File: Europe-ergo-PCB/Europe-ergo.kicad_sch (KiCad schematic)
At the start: 230 parts, among them J1 Conn_01x04_Male/I2C, J2 Conn_01x04_Male, SW1 MX-NO-LED, SW10 MX-NO-LED, SW11 MX-NO-LED, SW12 MX-NO-LED, SW13 MX-NO-LED, SW14 MX-NO-LED, SW15 MX-NO-LED, SW16 MX-NO-LED, SW17 MX-NO-LED, SW18 MX-NO-LED, SW19 MX-NO-LED, SW2 MX-NO-LED, SW20 MX-NO-LED, SW21 MX-NO-LED, SW22 MX-NO-LED, SW23 MX-NO-LED, SW24 MX-NO-LED, SW25 MX-NO-LED, SW26 MX-NO-LED, SW27 MX-NO-LED, SW28 MX-NO-LED, SW29 MX-NO-LED, SW3 MX-NO-LED, SW30 MX-NO-LED, SW31 MX-NO-LED, SW32 MX-NO-LED, SW33 MX-NO-LED, SW34 MX-NO-LED, SW35 MX-NO-LED, SW36 MX-NO-LED, SW37 MX-NO-LED, SW38 MX-NO-LED, SW39 MX-NO-LED, SW4 MX-NO-LED, SW40 MX-NO-LED, SW41 MX-NO-LED, SW42 MX-NO-LED, SW43 MX-NO-LED, SW44 MX-NO-LED, SW45 MX-NO-LED, SW46 MX-NO-LED, SW47 MX-NO-LED, SW48 SW_Push, SW49 SW_Push, SW5 MX-NO-LED, SW50 MX-NO-LED, SW51 MX-NO-LED, SW52 MX-NO-LED, SW53 MX-NO-LED, SW54 MX-NO-LED, SW55 MX-NO-LED, SW56 MX-NO-LED, SW57 MX-NO-LED, SW58 MX-NO-LED, SW59 MX-NO-LED, SW6 MX-NO-LED, SW60 MX-NO-LED, SW61 MX-NO-LED, SW62 MX-NO-LED, SW63 MX-NO-LED, SW64 MX-NO-LED, SW65 MX-NO-LED, SW66 MX-NO-LED, SW67 MX-NO-LED, SW68 MX-NO-LED, SW69 MX-NO-LED, SW7 MX-NO-LED, SW70 MX-NO-LED, SW71 MX-NO-LED, SW72 MX-NO-LED, SW73 MX-NO-LED, SW74 MX-NO-LED, SW75 MX-NO-LED, SW76 MX-NO-LED, SW77 MX-NO-LED, SW78 MX-NO-LED, SW79 MX-NO-LED, SW8 MX-NO-LED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

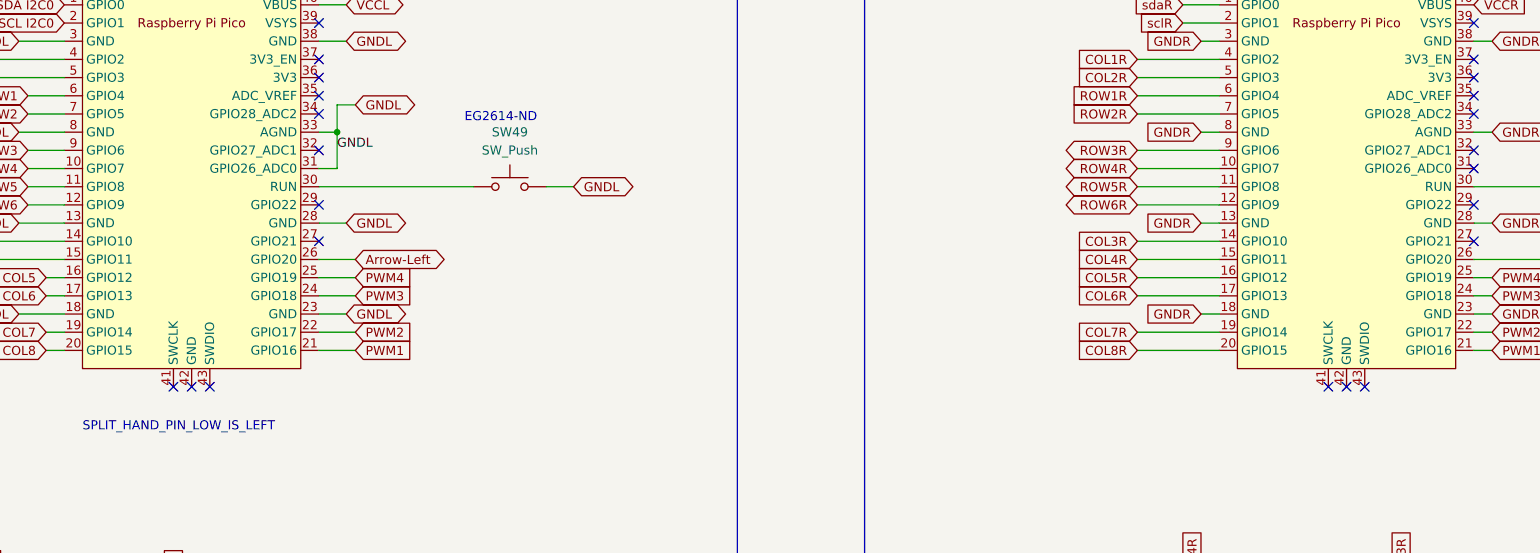
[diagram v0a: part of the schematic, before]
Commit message: Add files via upload
small fix
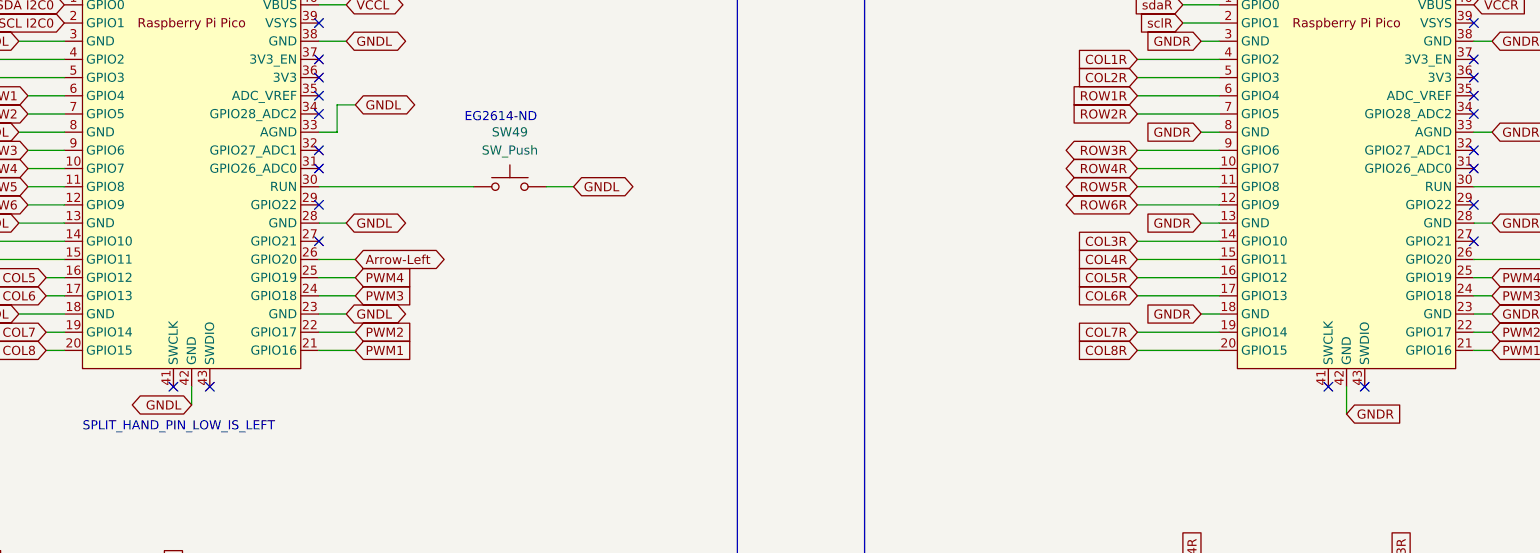
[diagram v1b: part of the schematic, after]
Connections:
- net GNDL: now also U2.42 (GND); no longer U2.31 (GPIO26_ADC0)
- net GNDR: now also U1.42 (GND)
- no-connect marks 23 -> 22
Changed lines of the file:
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@@
   (junction (at 722.63 241.3) (diameter 0) (color 0 0 0 0)
-  )
-  (junction (at 344.17 58.42) (diameter 0) (color 0 0 0 0)
   )
   (junction (at 759.46 223.52) (diameter 0) (color 0 0 0 0)
@@
   (no_connect (at 341.63 48.26))
   (no_connect (at 321.31 93.98))
-  (no_connect (at 323.85 93.98))
   (no_connect (at 502.92 48.26))
   (no_connect (at 502.92 53.34))
@@
   (no_connect (at 341.63 50.8))
   (no_connect (at 482.6 93.98))
-  (no_connect (at 485.14 93.98))
+  (no_connect (at 341.63 63.5))
   (no_connect (at 502.92 73.66))
   (no_connect (at 341.63 53.34))
@@
     (stroke (width 0) (type default) (color 0 0 0 0))
   )
-  (wire (pts (xy 341.63 63.5) (xy 344.17 63.5))
-    (stroke (width 0) (type default) (color 0 0 0 0))
-  )
   (wire (pts (xy 502.92 78.74) (xy 505.46 78.74))
     (stroke (width 0) (type default) (color 0 0 0 0))
@@
     (stroke (width 0) (type default) (color 0 0 0 0))
   )
-  (wire (pts (xy 344.17 58.42) (xy 344.17 63.5))
-    (stroke (width 0) (type default) (color 0 0 0 0))
-  )
   (wire (pts (xy 100.33 134.62) (xy 100.33 138.43))
     (stroke (width 0) (type default) (color 0 0 0 0))
@@
     (stroke (width 0) (type default) (color 0 0 0 0))
   )
+  (wire (pts (xy 485.14 93.98) (xy 485.14 97.79))
+    (stroke (width 0) (type default) (color 0 0 0 0))
+  )
   (wire (pts (xy 687.07 120.65) (xy 661.67 120.65))
     (stroke (width 0) (type default) (color 0 0 0 0))
@@
   )
   (wire (pts (xy 676.91 210.82) (xy 674.37 210.82))
+    (stroke (width 0) (type default) (color 0 0 0 0))
+  )
+  (wire (pts (xy 323.85 93.98) (xy 323.85 96.52))
     (stroke (width 0) (type default) (color 0 0 0 0))
   )
@@
     (effects (font (size 1.27 1.27)) (justify left bottom))
   )
-  (label "GNDL" (at 344.17 60.96 0)
-    (effects (font (size 1.27 1.27)) (justify left bottom))
-  )
   (label "RUN" (at 515.62 66.04 0)
     (effects (font (size 1.27 1.27)) (justify left bottom))
@@
     )
   )
+  (global_label "GNDR" (shape input) (at 485.14 97.79 0) (fields_autoplaced)
+    (effects (font (size 1.27 1.27)) (justify left))
+    (property "Intersheet References" "${INTERSHEET_REFS}" (id 0) (at 492.6047 97.7106 0)
+      (effects (font (size 1.27 1.27)) (justify left) hide)
+    )
+  )
   (global_label "VCCR" (shape input) (at 502.92 40.64 0) (fields_autoplaced)
     (effects (font (size 1.27 1.27)) (justify left))
@@
     )
   )
+  (global_label "GNDL" (shape bidirectional) (at 323.85 96.52 180) (fields_autoplaced)
+    (effects (font (size 1.27 1.27)) (justify right))
+    (property "Intersheet References" "${INTERSHEET_REFS}" (id 0) (at 316.5383 96.4406 0)
+      (effects (font (size 1.27 1.27)) (justify right) hide)
+    )
+  )

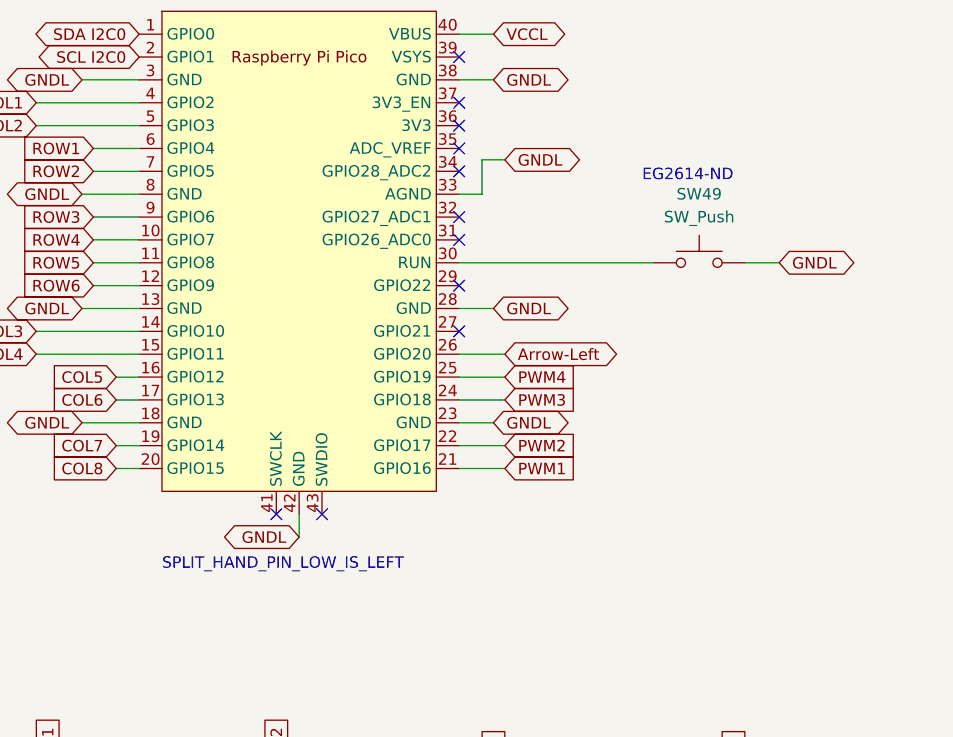
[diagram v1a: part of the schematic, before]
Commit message: Add files via upload
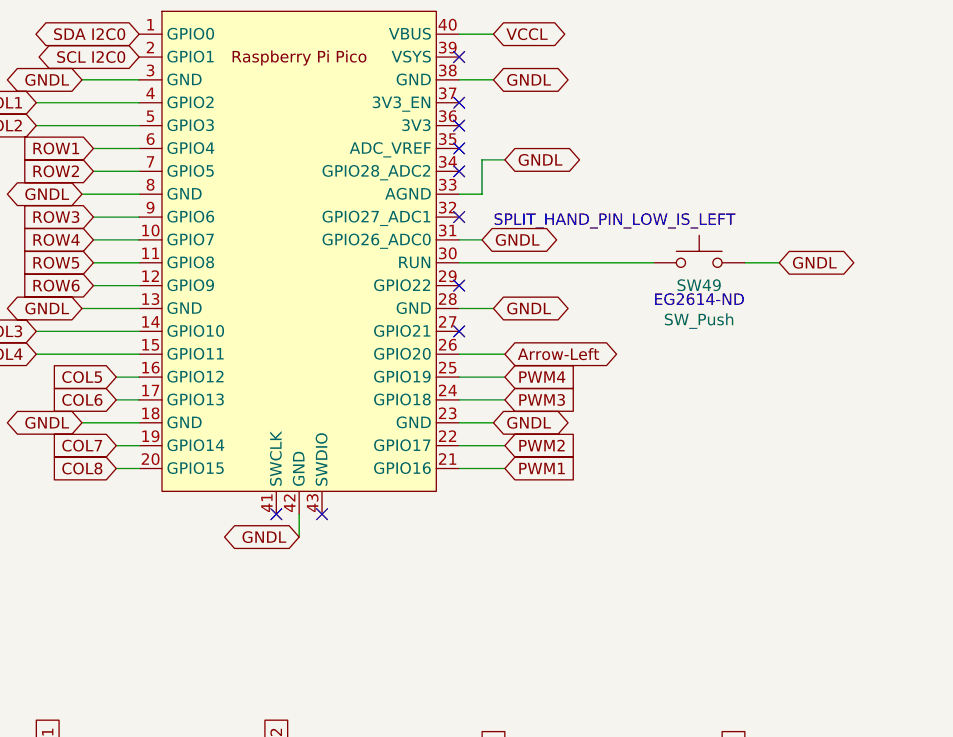
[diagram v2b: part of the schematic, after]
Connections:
- net GNDL: now also U2.31 (GPIO26_ADC0)
- no-connect marks 22 -> 21
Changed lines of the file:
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@@
   (no_connect (at 341.63 50.8))
   (no_connect (at 482.6 93.98))
-  (no_connect (at 341.63 63.5))
   (no_connect (at 502.92 73.66))
   (no_connect (at 341.63 53.34))
@@
     (stroke (width 0) (type default) (color 0 0 0 0))
   )
+  (wire (pts (xy 341.63 63.5) (xy 344.17 63.5))
+    (stroke (width 0) (type default) (color 0 0 0 0))
+  )
   (wire (pts (xy 651.51 100.33) (xy 651.51 138.43))
     (stroke (width 0) (type default) (color 0 0 0 0))
@@
     (stroke (width 0) (type default) (color 0 0 0 0))
   )
-  (text "EG2614-ND" (at 361.95 57.15 0)
+  (text "EG2614-ND" (at 363.22 71.12 0)
     (effects (font (size 1.27 1.27)) (justify left bottom))
   )
@@
     (effects (font (size 1.27 1.27)) (justify left bottom))
   )
-  (text "SPLIT_HAND_PIN_LOW_IS_LEFT" (at 308.61 100.33 0)
+  (text "SPLIT_HAND_PIN_LOW_IS_LEFT" (at 345.44 62.23 0)
     (effects (font (size 1.27 1.27)) (justify left bottom))
   )
@@
     )
   )
+  (global_label "GNDL" (shape bidirectional) (at 344.17 63.5 0) (fields_autoplaced)
+    (effects (font (size 1.27 1.27)) (justify left))
+    (property "Intersheet References" "${INTERSHEET_REFS}" (id 0) (at 351.4817 63.5794 0)
+      (effects (font (size 1.27 1.27)) (justify left) hide)
+    )
+  )
   (global_label "VCCR" (shape input) (at 513.08 196.85 0) (fields_autoplaced)
     (effects (font (size 1.27 1.27)) (justify left))
@@
   )
   (symbol (lib_id "Switch:SW_Push") (at 368.3 66.04 0) (unit 1)
-    (in_bom yes) (on_board yes) (fields_autoplaced)
-    (property "Reference" "SW49" (id 0) (at 368.3 58.42 0))
-    (property "Value" "SW_Push" (id 1) (at 368.3 60.96 0))
+    (in_bom yes) (on_board yes)
+    (property "Reference" "SW49" (id 0) (at 368.3 68.58 0))
+    (property "Value" "SW_Push" (id 1) (at 368.3 72.39 0))
     (property "Footprint" "switch:switch_P5.08mm" (id 2) (at 368.3 60.96 0)
       (effects (font (size 1.27 1.27)) hide)

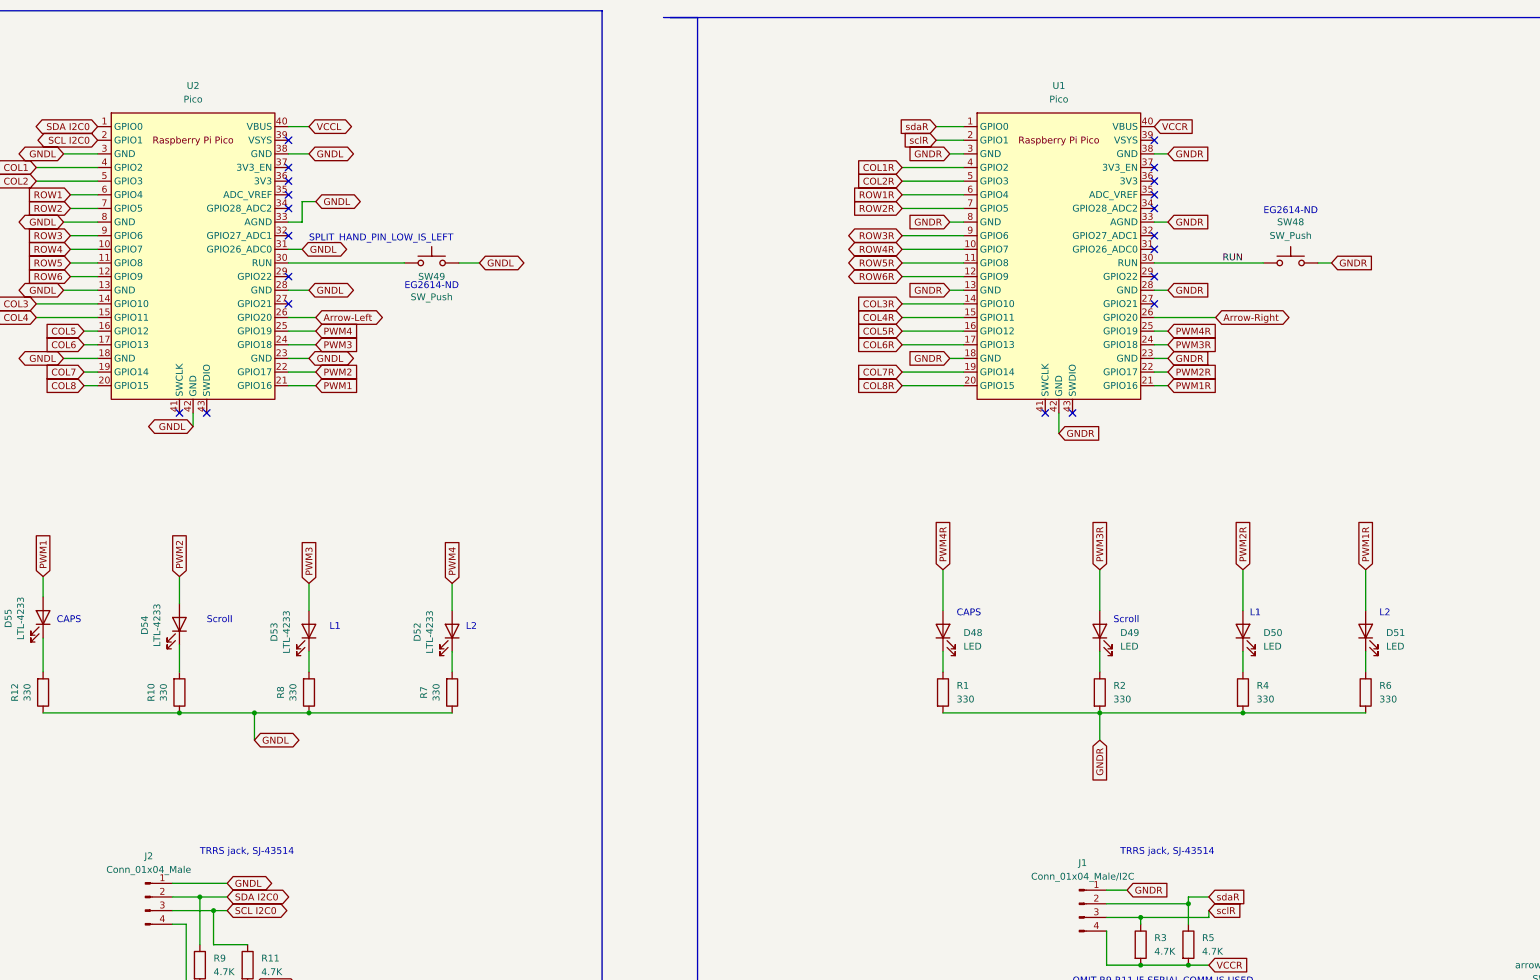
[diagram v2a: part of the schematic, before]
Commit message: Add files via upload
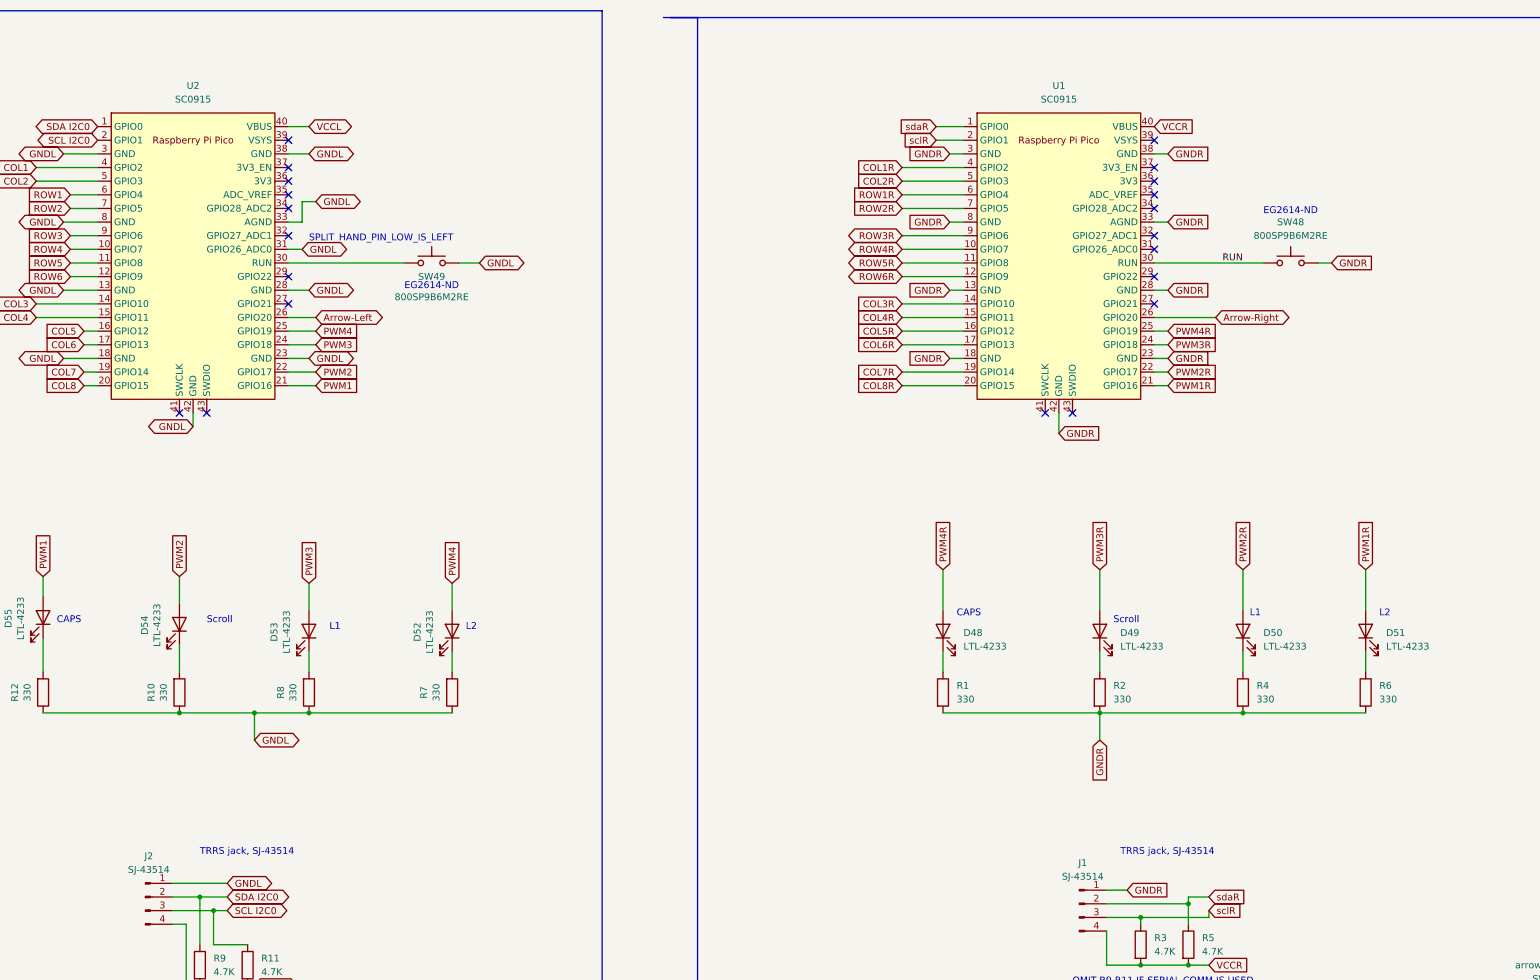
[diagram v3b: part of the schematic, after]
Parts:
- D48, D49, D50, D51: value LED -> LTL-4233
- J1: value Conn_01x04_Male/I2C -> SJ-43514
- J2: value Conn_01x04_Male -> SJ-43514
- SW1, SW10, SW11, SW12, SW13, SW14, SW15, SW16, SW17, SW18, SW19, SW2, SW20, SW21, SW22, SW23, SW24, SW25, SW26, SW27, SW28, SW29, SW3, SW30, SW31, SW32, SW33, SW34, SW35, SW36, SW37, SW38, SW39, SW4, SW40, SW41, SW42, SW43, SW44, SW45, SW46, SW47, SW5, SW50, SW51, SW52, SW53, SW54, SW55, SW56, SW57, SW58, SW59, SW6, SW60, SW61, SW62, SW63, SW64, SW65, SW66, SW67, SW68, SW69, SW7, SW70, SW71, SW72, SW73, SW74, SW75, SW76, SW77, SW78, SW79, SW8, SW80, SW81, SW82, SW83, SW84, SW85, SW86, SW87, SW88, SW89, SW9, SW90, SW91, SW92, SW93, SW94, SW95, SW96: value MX-NO-LED -> MX1A-G1NN
- SW48, SW49: value SW_Push -> 800SP9B6M2RE
- U1, U2: value Pico -> SC0915
